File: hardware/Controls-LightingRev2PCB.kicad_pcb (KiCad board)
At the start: 2 copper layers, 53.5 x 53.5 mm, 52 parts, among them IC1 LM74502HDDFR, IC3 ACS724LLCTR-05AU-T, IC4 ACS724LLCTR-05AU-T, IC5 TLV70433DBVT, IC6 ACS724LLCTR-05AU-T, J1 53307-2471, J3 Conn_02x05_Top_Bottom, J4 Conn_01x02, J5 Conn_01x02, J6 Conn_01x03, Q1 NVMFWS1D7N04XMT1G, Q3 IRLML0030, Q4 NVMFWS1D7N04XMT1G, Q5 IRLML0030, U5 SN74LV1T34DBV

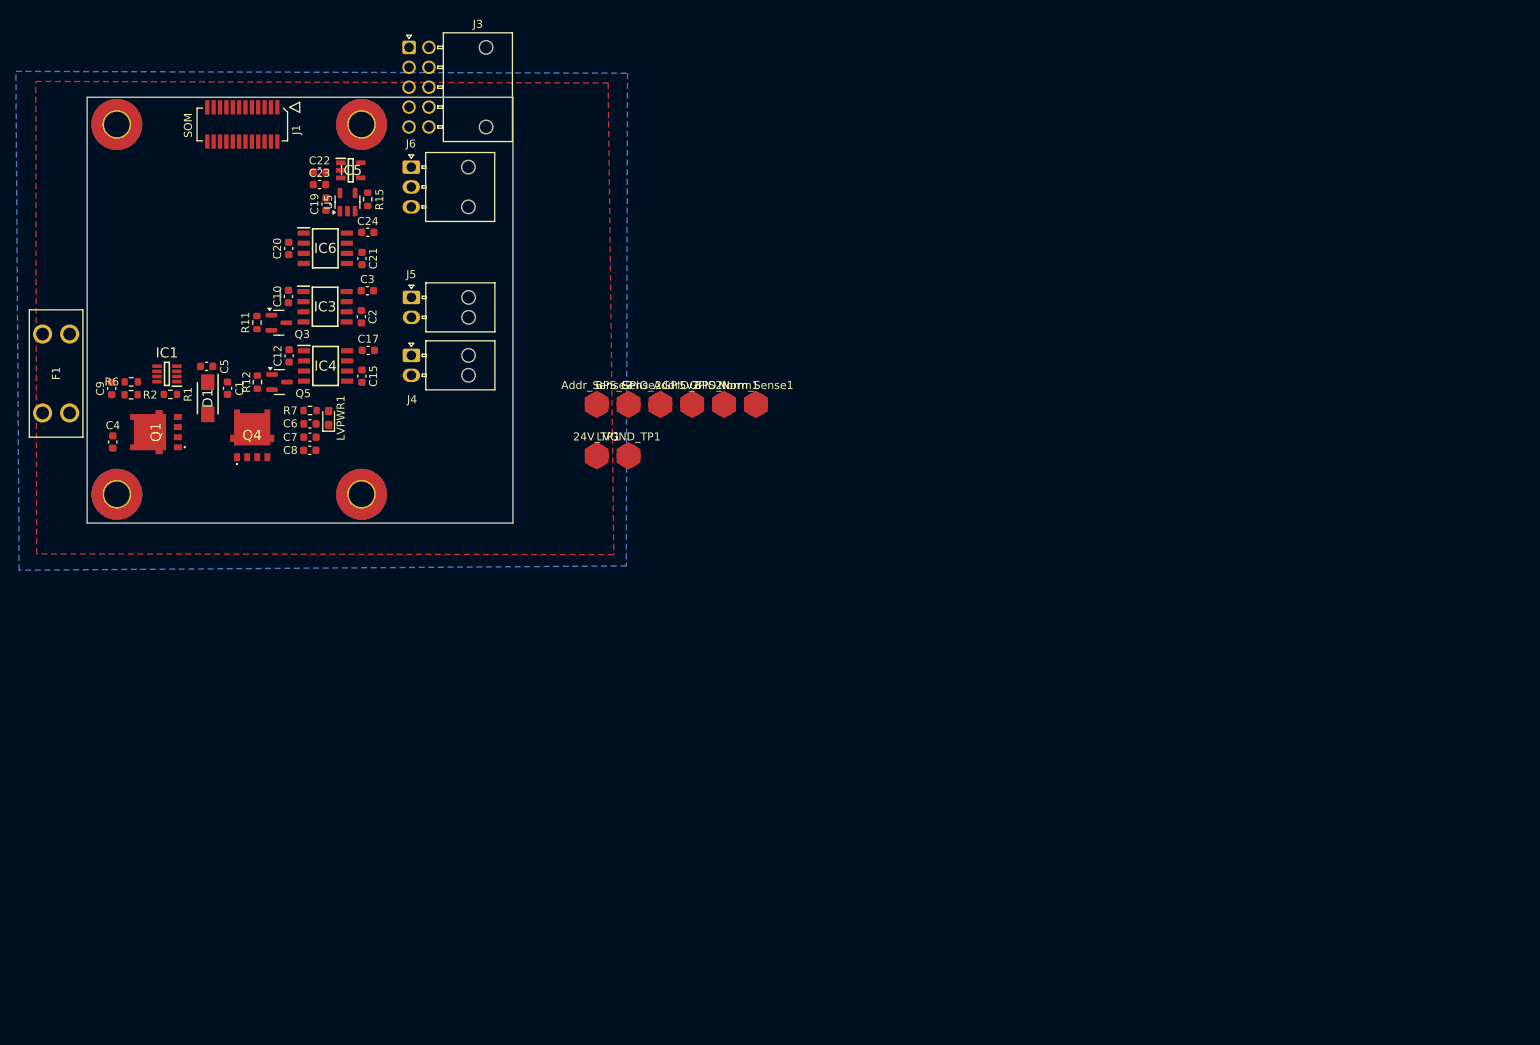
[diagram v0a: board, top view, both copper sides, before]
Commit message: layout recommendations
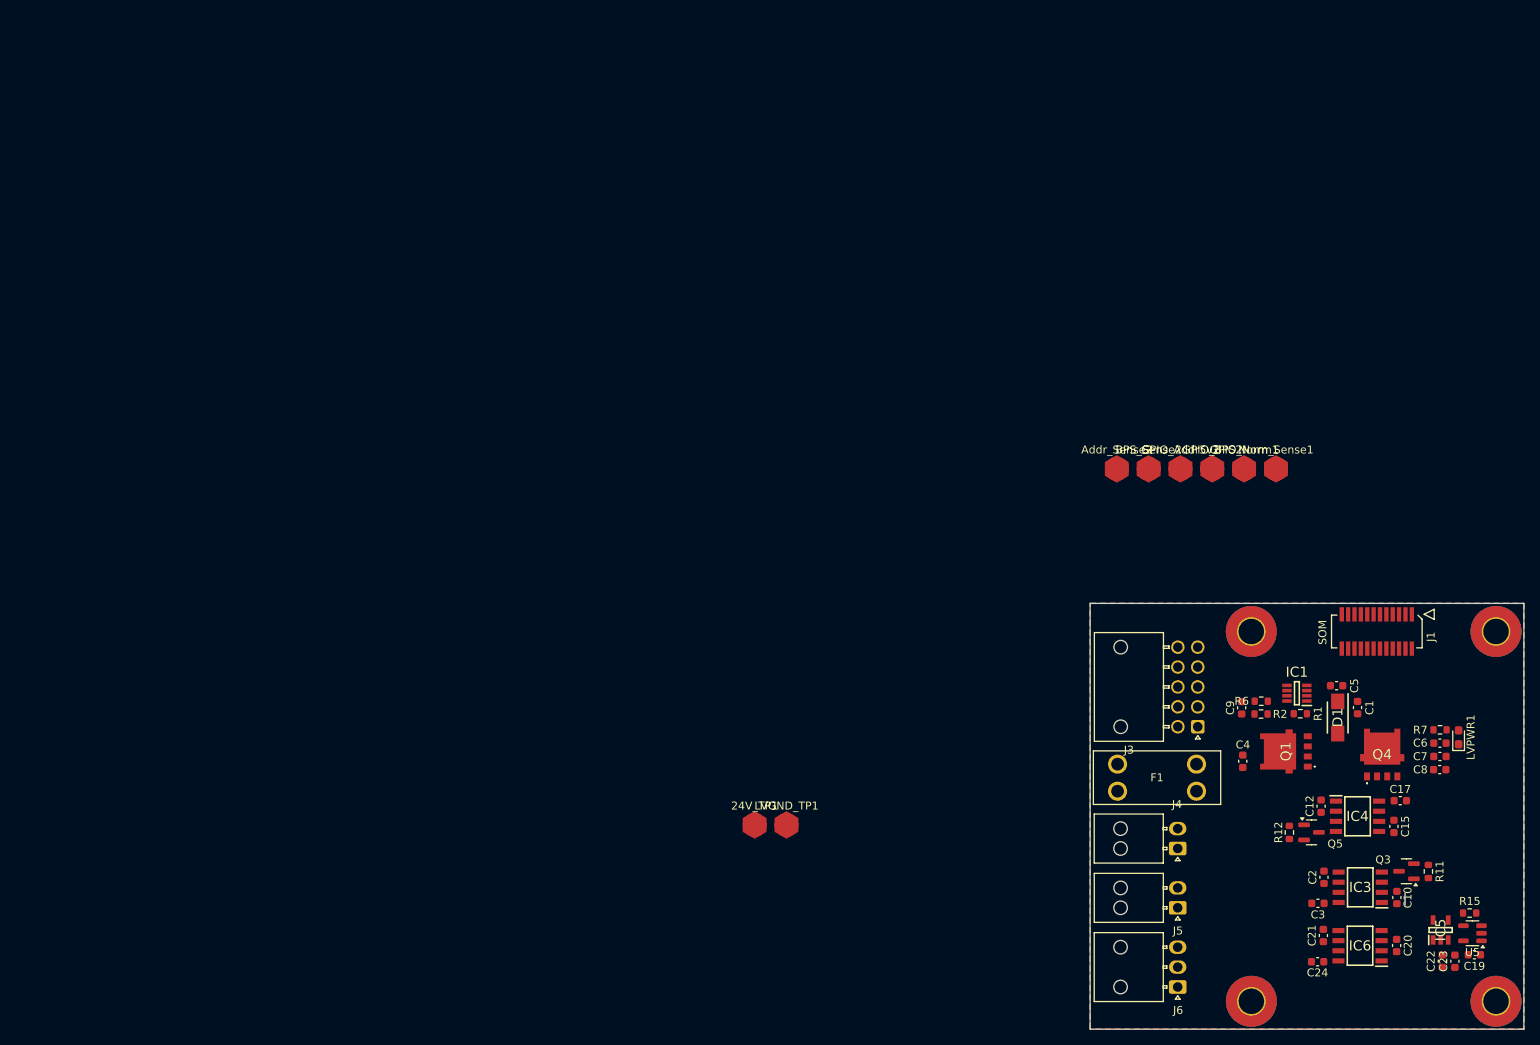
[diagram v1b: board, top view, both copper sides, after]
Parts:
- moved C23 172.8 mm to (219.8, 130.0), turned to 90 degrees
- moved C22 172.4 mm to (218.3, 130.0), turned to 90 degrees
- moved C19 172.4 mm to (222.3, 129.2), turned to 180 degrees
- moved U5 168.6 mm to (222.0, 126.5), turned to 180 degrees
- moved IC5 166.9 mm to (218.0, 126.0), turned to 90 degrees
- moved R15 165.0 mm to (221.7, 123.9), turned to 180 degrees
- moved C20 164.5 mm to (212.5, 128.0), turned to -90 degrees
- moved R11 162.6 mm to (216.5, 118.7), turned to -90 degrees
- moved C10 158.4 mm to (212.5, 122.0), turned to 90 degrees
- moved Q3 157.6 mm to (213.7, 118.7), turned to 180 degrees
- moved IC6 156.8 mm to (207.9, 128.0), turned to 180 degrees
- moved J1 156.1 mm to (210.0, 88.5)
- moved C24 150.5 mm to (202.6, 130.0), turned to 180 degrees
- moved IC3 149.1 mm to (207.9, 120.7), turned to 180 degrees
- moved C21 147.8 mm to (203.3, 126.7), turned to 90 degrees
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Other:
- board size 53.5 x 53.5 mm -> 54.5 x 53.5 mm
